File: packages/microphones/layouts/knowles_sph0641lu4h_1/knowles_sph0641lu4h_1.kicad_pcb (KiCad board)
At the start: 2 copper layers, 1 part

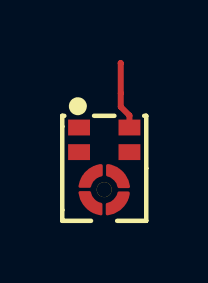
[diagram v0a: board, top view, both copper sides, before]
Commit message: review tool updates
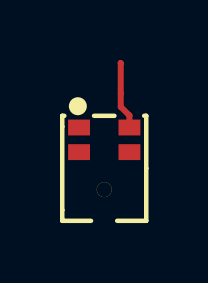
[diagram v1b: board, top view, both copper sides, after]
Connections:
- net GND renamed lv
- net VCC renamed hv
- U1 pad : net -> (no net)
